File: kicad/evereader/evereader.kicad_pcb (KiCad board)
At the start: 2 copper layers, 92 x 132 mm, 60 parts, among them J1 USB_C_Receptacle_USB2.0_14P, J2 Micro_SD_Card_Det1, J3 Conn_02x04_Odd_Even, J4 Conn_02x04_Odd_Even, J5 Conn_01x02, J6 Conn_01x08, J7 Conn_01x08, J8 Conn_01x02, J9 Conn_01x02, Q1 FS8205A, SW1 SW_Push, SW2 SW_Push, SW3 SW_Push, SW4 SW_Push, SW5 SW_Push, U1 TP4056-42-ESOP8, U2 DW01A, U3 AP2112K-3.3, U5 ESP32-S3-WROOM-1

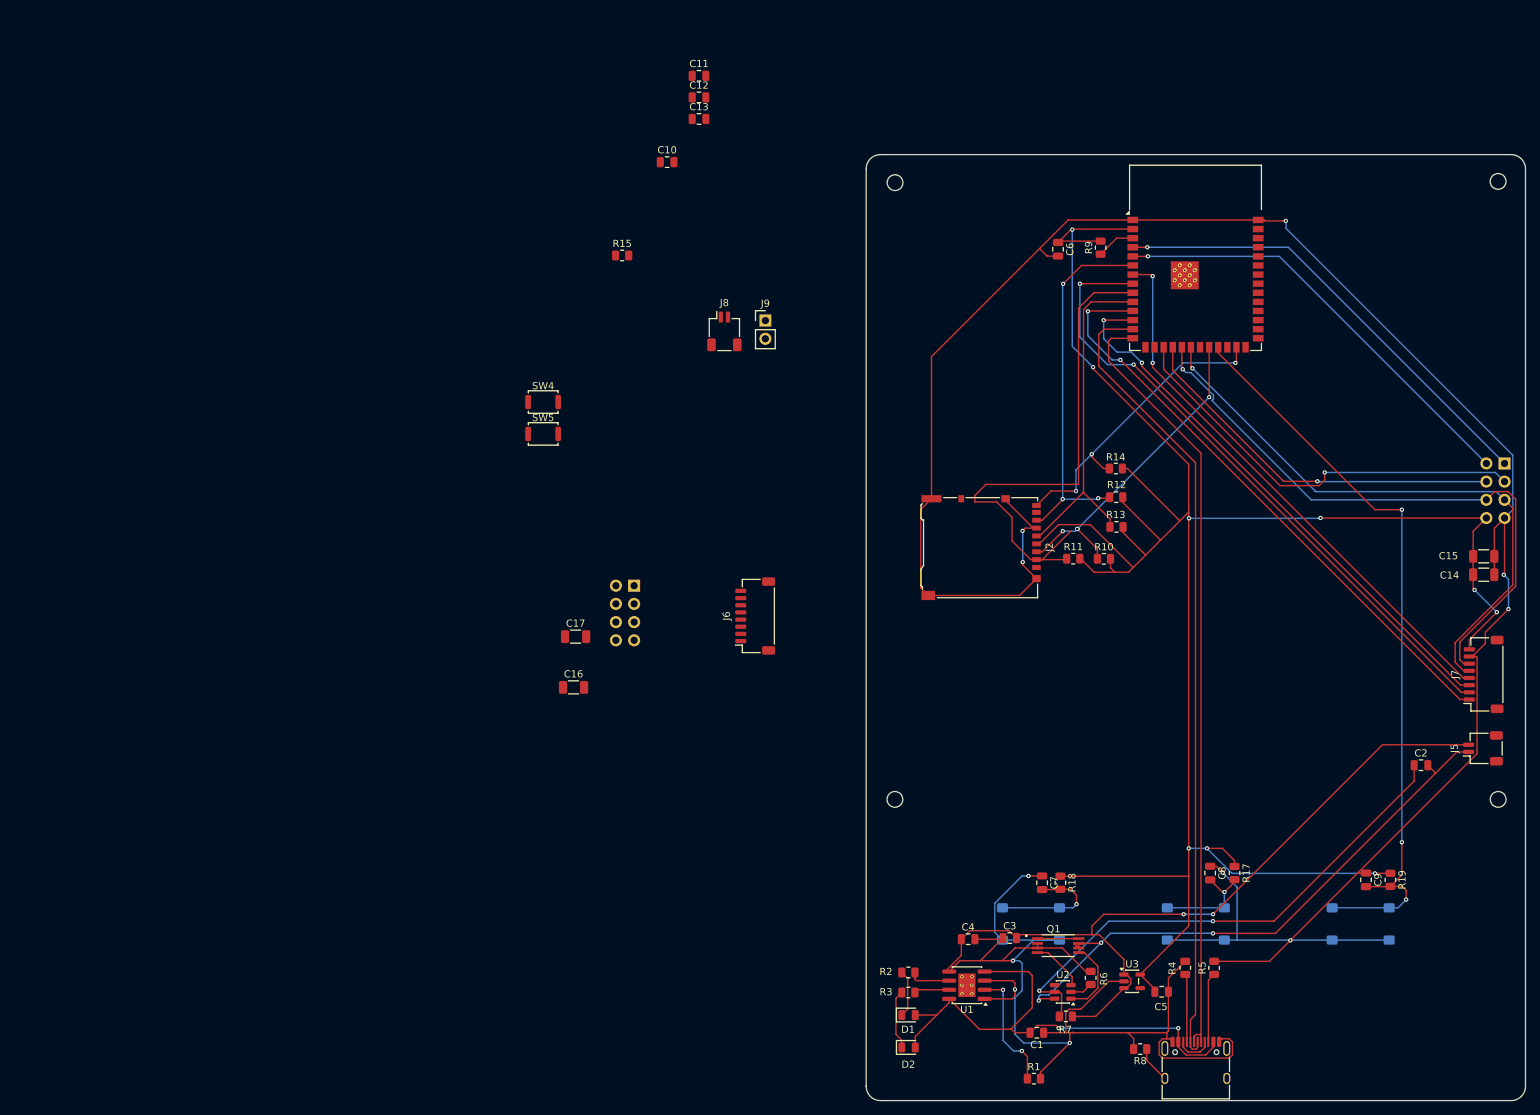
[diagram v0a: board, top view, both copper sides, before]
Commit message: finished the PCB, finally
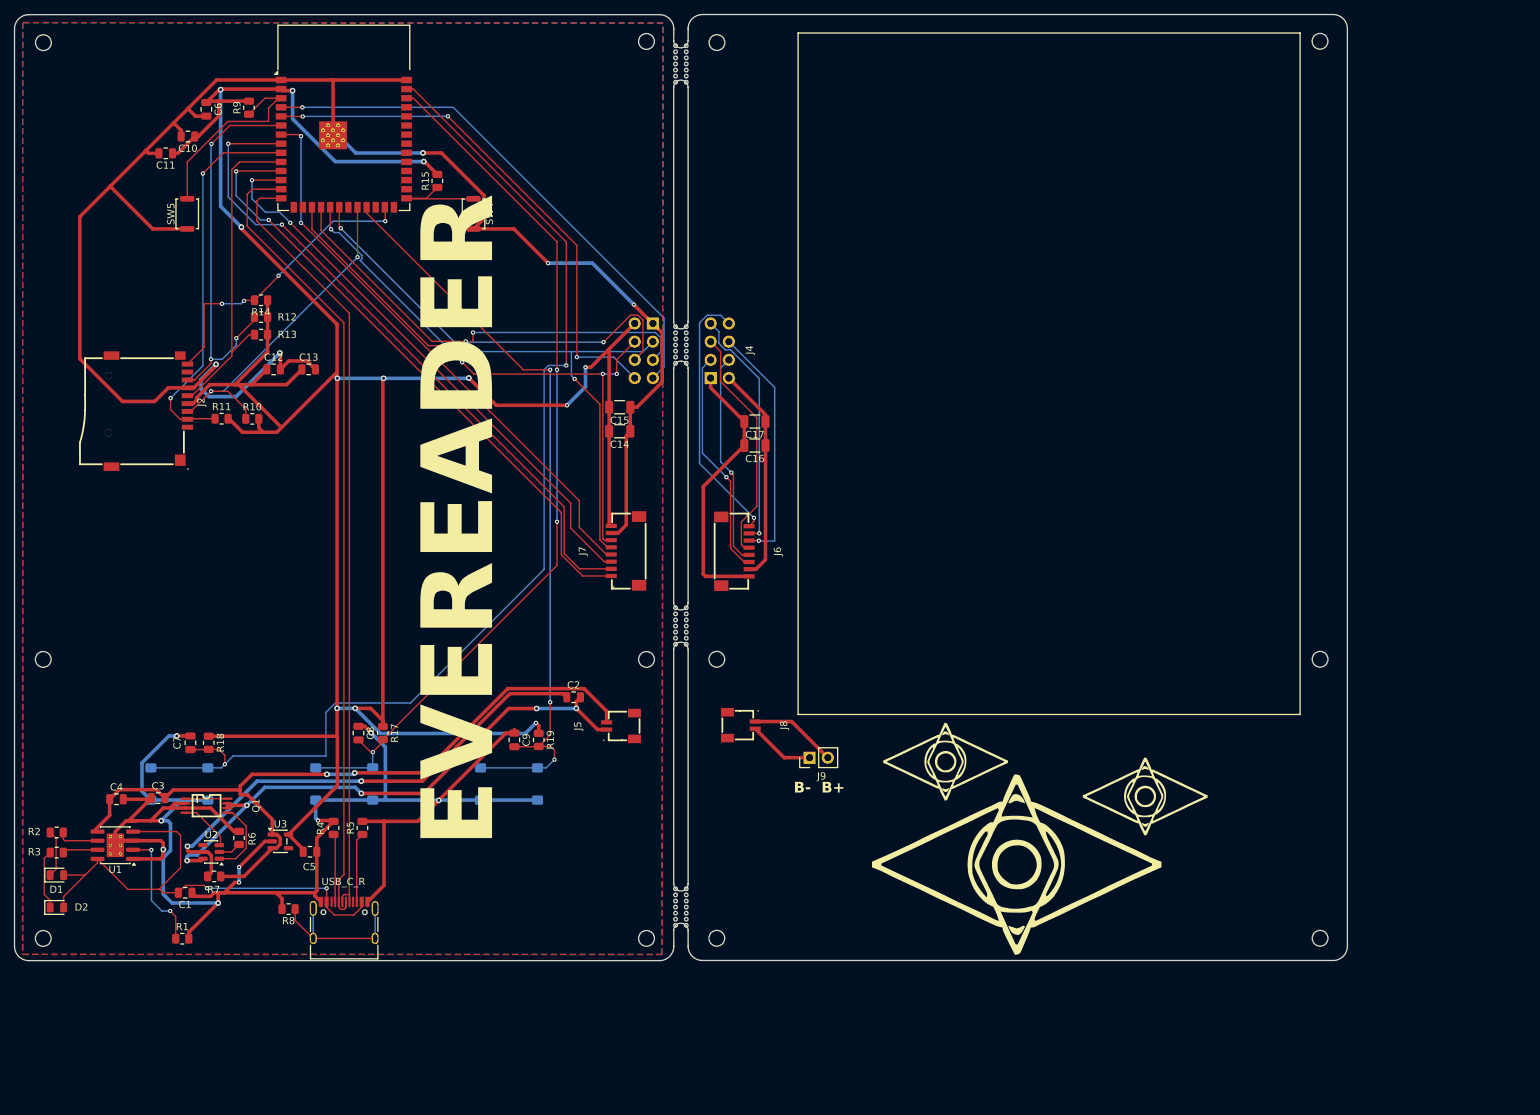
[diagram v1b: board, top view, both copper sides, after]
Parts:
- added REF**: MountingHole_2.2mm_M2, MountingHole:MountingHole_2.2mm_M2, F.Cu at (133.2, 117.6)
- added REF**: MountingHole_2.2mm_M2, MountingHole:MountingHole_2.2mm_M2, F.Cu at (133.2, 156.6)
- added REF**: MountingHole_2.2mm_M2, MountingHole:MountingHole_2.2mm_M2, F.Cu at (133.2, 31.6)
- added REF**: MouseBite-Slot_2.0x4.5mm_outset_D0.5mm_P0.85mm_7h, Panelization:MouseBite-Slot_2.0x4.5mm_outset_D0.5mm_P0.85mm_7h, F.Cu at (129.2, 152.2)
- added REF**: MountingHole_2.2mm_M2, MountingHole:MountingHole_2.2mm_M2, F.Cu at (217.3, 117.6)
- added REF**: MouseBite-Slot_2.0x4.5mm_outset_D0.5mm_P0.85mm_7h, Panelization:MouseBite-Slot_2.0x4.5mm_outset_D0.5mm_P0.85mm_7h, F.Cu at (129.2, 73.8)
- added REF**: MountingHole_2.2mm_M2, MountingHole:MountingHole_2.2mm_M2, F.Cu at (217.3, 31.4)
- added REF**: MouseBite-Slot_2.0x4.5mm_outset_D0.5mm_P0.85mm_7h, Panelization:MouseBite-Slot_2.0x4.5mm_outset_D0.5mm_P0.85mm_7h, F.Cu at (129.2, 34.5)
- added REF**: MouseBite-Slot_2.0x4.5mm_outset_D0.5mm_P0.85mm_7h, Panelization:MouseBite-Slot_2.0x4.5mm_outset_D0.5mm_P0.85mm_7h, F.Cu at (129.2, 113.0)
- added REF**: MountingHole_2.2mm_M2, MountingHole:MountingHole_2.2mm_M2, F.Cu at (217.3, 156.6)
- added REF**: MountingHole_2.2mm_M2, MountingHole:MountingHole_2.2mm_M2, F.Cu at (123.4, 156.6)
- added REF**: MountingHole_2.2mm_M2, MountingHole:MountingHole_2.2mm_M2, F.Cu at (39.2, 156.6)
- C1, C10, C12, C3, C4: value 10µF -> C15850
- C5, C6: value 1µF -> C28323
- J1: value USB_C_Receptacle_USB2.0_14P -> C165948
- J2: value Micro_SD_Card_Det1 -> C720505; footprint Connector_Card:microSD_HC_Hirose_DM3AT-SF-PEJM5 -> EasyEDA:TF-SMD_TF-115-BCP9
- J3, J4: value Conn_02x04_Odd_Even -> ~
- J5, J8: value Conn_01x02 -> C160402; footprint Connector_JST:JST_SH_SM02B-SRSS-TB_1x02-1MP_P1.00mm_Horizontal -> EasyEDA:CONN-SMD_2P-P1.00_SM02B-SRSS-TB-LF-SN
- J6, J7: value Conn_01x08 -> C160407; footprint Connector_JST:JST_SH_SM08B-SRSS-TB_1x08-1MP_P1.00mm_Horizontal -> EasyEDA:CONN-TH_SM08B-SRSS-TB-LF-SN
- J9: value Conn_01x02 -> ~
- Q1: value FS8205A -> C7525054; footprint FS8205A:SOP65P640X120-8N -> EasyEDA:TSSOP-8_L4.4-W3.0-P0.65-LS6.4-BL
- SW4, SW5: value SW_Push -> C139797
- U5: value ESP32-S3-WROOM-1 -> ESP32-S3-WROOM-1-N16-R8
- moved R13 122.3 mm to (69.6, 72.3)
- moved C15 122.3 mm to (119.6, 82.5)
- moved C14 122.2 mm to (119.6, 85.8)
- moved R12 121.9 mm to (69.6, 69.9)
- moved R14 121.6 mm to (69.6, 67.5)
- moved J7 121.0 mm to (120.4, 102.5)
- moved C6 120.4 mm to (61.9, 40.9)
- moved C7 120.4 mm to (59.7, 129.3)
- moved J3 120.4 mm to (124.2, 70.8)
- moved R10 120.4 mm to (68.3, 84.1)
- moved R11 120.4 mm to (64.1, 84.0)
- moved R17 120.4 mm to (86.6, 127.9)
- moved R19 120.4 mm to (108.3, 128.9)
- moved R4 120.4 mm to (79.7, 141.1)
- moved R5 120.4 mm to (83.7, 141.1)
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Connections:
- C16 pad 1: GND -> Net-(J4-Pin_2)
- C16 pad 2: Net-(J4-Pin_7) -> Net-(J4-Pin_1)
- C17 pad 1: GND -> Net-(J4-Pin_2)
- C17 pad 2: Net-(J4-Pin_7) -> Net-(J4-Pin_1)
- J3 pad 1: Net-(J3-Pin_1) -> GND
- J3 pad 2: Net-(J3-Pin_2) -> +3.3V
- J3 pad 7: GND -> Net-(J3-Pin_7)
- J3 pad 8: +3.3V -> Net-(J3-Pin_8)
- J6 pad 1: Net-(J4-Pin_1) -> Net-(J4-Pin_8)
- J6 pad 2: Net-(J4-Pin_2) -> Net-(J4-Pin_7)
- J6 pad 3: Net-(J4-Pin_3) -> Net-(J4-Pin_6)
- J6 pad 4: Net-(J4-Pin_4) -> Net-(J4-Pin_5)
- J6 pad 5: Net-(J4-Pin_5) -> Net-(J4-Pin_4)
- J6 pad 6: Net-(J4-Pin_6) -> Net-(J4-Pin_3)
- J6 pad 7: Net-(J4-Pin_7) -> Net-(J4-Pin_2)
- J6 pad 8: Net-(J4-Pin_8) -> Net-(J4-Pin_1)
- J7 pad 5: Net-(J3-Pin_5) -> Net-(J3-Pin_3)
- J7 pad 6: Net-(J3-Pin_6) -> Net-(J3-Pin_4)
- J9 pad 1: Net-(J8-Pin_1) -> Net-(J8-Pin_2)
- J9 pad 2: Net-(J8-Pin_2) -> Net-(J8-Pin_1)
- SW5 pad 2: +3.3V -> Net-(U5-EN)
- U1 pad 9: unconnected-(U1-EPAD-Pad9) -> GND
- U5 pad 17: Net-(J3-Pin_3) -> Net-(J3-Pin_5)
- U5 pad 18: Net-(J3-Pin_4) -> Net-(J3-Pin_6)
- U5 pad 19: Net-(J3-Pin_6) -> Net-(J3-Pin_4)
- U5 pad 20: Net-(J3-Pin_5) -> Net-(J3-Pin_3)
- U5 pad 4: Net-(J3-Pin_1) -> Net-(J3-Pin_7)
- U5 pad 5: Net-(J3-Pin_2) -> Net-(J3-Pin_8)
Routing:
- net Net-(U5-IO1): track 16.9 -> 155.9 mm, vias 1 -> 2
- net Net-(U5-IO2): track 16.3 -> 124.6 mm, vias 1 -> 3
- net +3.3V: track 314.0 -> 415.7 mm, vias 9 -> 12
- net Net-(J3-Pin_7): track 0.00 -> 74.6 mm, vias 0 -> 1
- net Net-(J3-Pin_8): track 0.00 -> 73.7 mm, vias 0 -> 3
- net Net-(J3-Pin_1): track 64.4 -> 0.00 mm, vias 1 -> 0
- net Net-(J3-Pin_2): track 61.3 -> 0.00 mm, vias 1 -> 0
- net Net-(J4-Pin_1): track 0.00 -> 38.2 mm
- net Net-(J4-Pin_8): track 0.00 -> 36.8 mm, vias 0 -> 1
- net Net-(J4-Pin_6): track 0.00 -> 34.1 mm, vias 0 -> 1
- net Net-(J4-Pin_7): track 0.00 -> 33.9 mm, vias 0 -> 1
- net Net-(J4-Pin_5): track 0.00 -> 33.1 mm
- net Net-(J4-Pin_3): track 0.00 -> 31.8 mm, vias 0 -> 1
- net Net-(J4-Pin_2): track 0.00 -> 30.3 mm
- net Net-(J4-Pin_4): track 0.00 -> 29.9 mm, vias 0 -> 1
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- added copper zone on B.Cu, net GND
- added copper zone on F.Cu, net GND
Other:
- board size 92 x 132 mm -> 186 x 132 mm
- board text added: "B- B+"
- board text added: "EVEREADER"
- board text added: "USB_C_R"
